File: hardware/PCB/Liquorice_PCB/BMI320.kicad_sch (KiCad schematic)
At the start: 8 parts, among them U1 BMI320, U3 XC6206PxxxMR

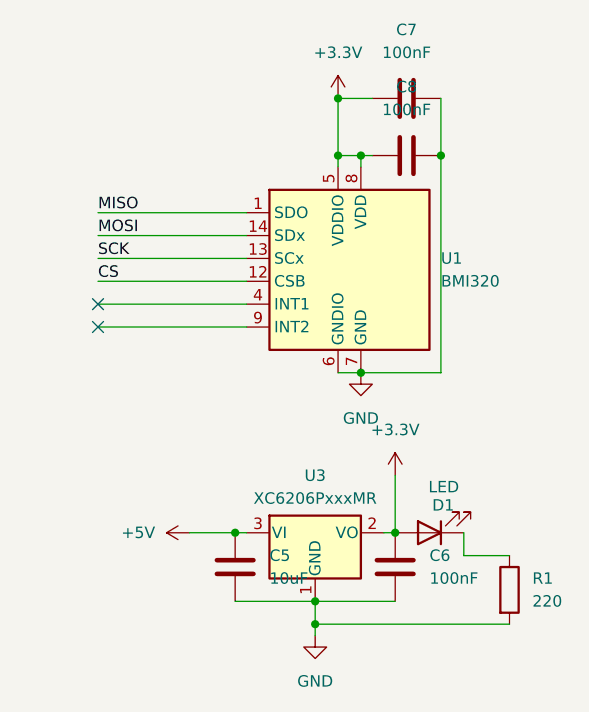
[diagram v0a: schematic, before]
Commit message: Added BOM and finialized main schematic.
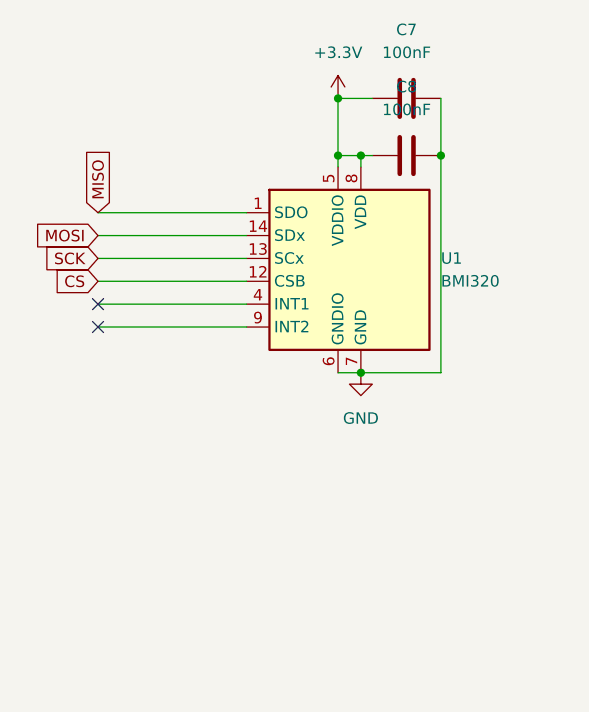
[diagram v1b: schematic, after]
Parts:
- removed C5: 10uF, Capacitor_SMD:C_0805_2012Metric_Pad1.18x1.45mm_HandSolder, symbol Device:C
- removed C6: 100nF, Capacitor_SMD:C_0805_2012Metric_Pad1.18x1.45mm_HandSolder, symbol Device:C
- removed D1: LED, LED_SMD:LED_0603_1608Metric_Pad1.05x0.95mm_HandSolder, symbol Device:LED
- removed R1: 220, Resistor_SMD:R_0603_1608Metric_Pad0.98x0.95mm_HandSolder, symbol Device:R
- removed U3: XC6206PxxxMR, Package_TO_SOT_SMD:SOT-23-3, symbol Regulator_Linear:XC6206PxxxMR
